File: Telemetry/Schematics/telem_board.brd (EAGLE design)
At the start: 39.9 x 66 mm, 30 parts, among them IC1 PIC18F26K80I/SP, IC2 PTN78000WAH, IC3 ISO1050DUB, IC4 FT232RL, J1 ICD, J2 TELEM, J3 TELEM, J4 TEMP SENSOR, J5 HALL SENSOR, Q4 20M, X1 PN61729-S, X2 +12V

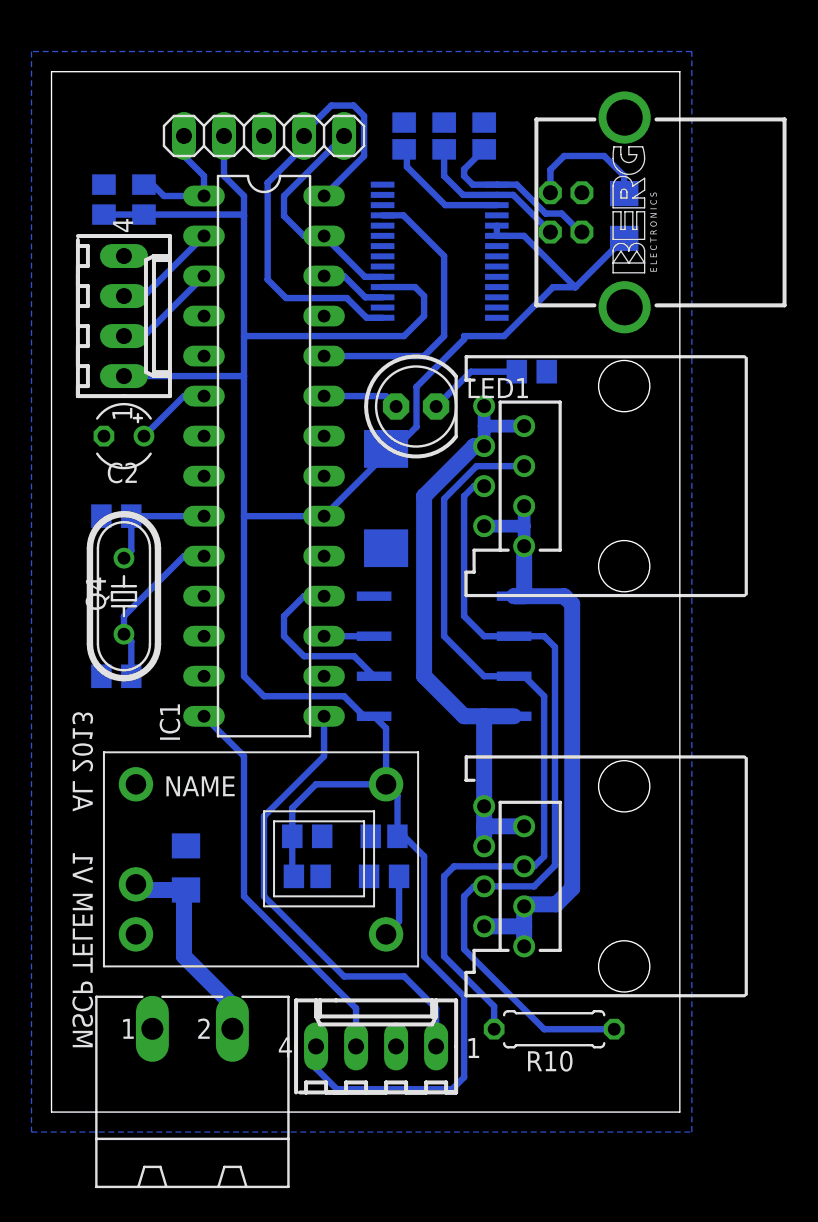
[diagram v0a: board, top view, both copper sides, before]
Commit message: v2
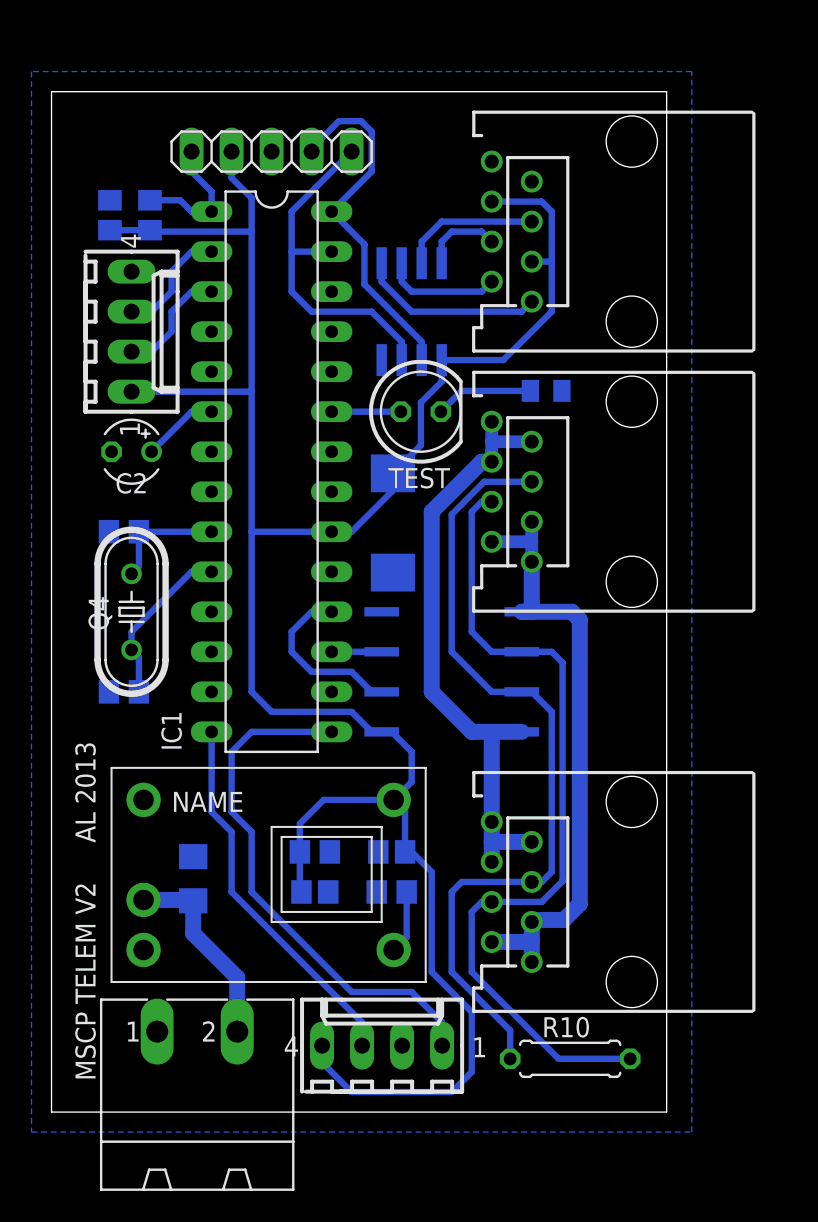
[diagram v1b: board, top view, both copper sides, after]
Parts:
- removed C10: 100n, resistor:C0805
- removed C3, C8: 47p, resistor:C0805
- removed F1: 0.5, MSCP_2011_v2:F1206
- removed LED1: (no value), adafruit:LED5MM
- removed X2: +12V, con-phoenix-508:MSTBA2
- added J7: RADIO, con-amp:215877-7
- added TEST: (no value), led:LED5MM
- IC4: value FT232RL -> SN75LBC179D; device MSCP_2011_v2:SSOP28 -> MSCP_2011_v1:SO08
- J2, J3: value TELEM -> CANBUS
- R2: device rcl:R0805 -> adafruit:R0805
- X1: value PN61729-S -> +12V; device con-berg:PN61729-S -> con-phoenix-508:MSTBA2
- moved X1 63.2 mm to (9.25, 0.03), turned to 0 degrees
- moved IC4 4.23 mm to (22.9, 50.8), turned to 0 degrees
- moved R10 2.14 mm to (32.9, 3.38)
- moved C4 1.61 mm to (21.7, 37.4)
- moved R2 1.52 mm to (31.4, 45.8), turned to 0 degrees
- moved IC1 1.10 mm to (14.0, 40.6)
- moved J1 1.10 mm to (14.0, 61.0)
- moved C7 1.10 mm to (4.60, 36.8)
- moved C2 1.10 mm to (5.08, 41.9)
- moved J4 1.10 mm to (5.08, 49.5)
- moved Q4 1.10 mm to (5.08, 31.8)
- moved C11 1.10 mm to (16.7, 14.0)
- moved IC2 1.10 mm to (14.0, 15.2)
- moved J2 1.10 mm to (36.8, 39.4)
- moved R1 1.10 mm to (21.6, 14.0)
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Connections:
- removed net N$9: C10.1, IC4.17
- new net N$12: IC4.5, J7.1
- net +12V: now also X1.2; no longer X2.2
- net +5V: now also IC4.1, J7.3, J7.6; no longer F1.1, IC4.19, IC4.20, IC4.4
- net CTS: no longer IC4.11
- net GND: now also IC4.4, J7.7, J7.8, R2.1, X1.1; no longer C10.2, C3.2, C8.2, IC4.18, IC4.21, IC4.25, IC4.26, IC4.7, R2.2, X1.4, X2.1
- net N$10: now also IC4.6, J7.2; no longer F1.2, X1.1
- net N$3: now also IC4.7, J7.5; no longer IC1.23, LED1.A
- net N$4: now also IC4.8, J7.4; no longer LED1.K, R2.1
- net N$6: now also IC1.23, TEST.A; no longer C8.1, IC4.16, X1.2
- net N$7: now also R2.2, TEST.K; no longer C3.1, IC4.15, X1.3
- net RTS: no longer IC4.3
- net RX: now also IC4.2; no longer IC4.1
- net TX: now also IC4.3; no longer IC4.5
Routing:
- net CTS: track 18.2 -> 0.00 mm
- net +5V: track 165.4 -> 148.7 mm
- net N$12: track 0.00 -> 11.7 mm
- net TX: track 14.5 -> 22.5 mm
- net N$9: track 7.90 -> 0.00 mm
- net RX: track 29.5 -> 22.9 mm
- net N$6: track 9.91 -> 4.39 mm
- net N$7: track 11.2 -> 6.23 mm
- net RTS: track 4.27 -> 0.00 mm
- net N$3: track 4.85 -> 8.88 mm
- net SDA: track 29.3 -> 33.3 mm
- net N$15: track 51.2 -> 52.3 mm
- net N$14: track 50.6 -> 51.8 mm
- net SCL: track 25.0 -> 23.9 mm
- net +12V: track 13.7 -> 12.6 mm
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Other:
- board size 39.9 x 66 mm -> 39 x 64.8 mm
- board text added: "MSCP TELEM V2 AL 2013"
- board text removed: "MSCP TELEM V1 AL 2013"

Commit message: v3
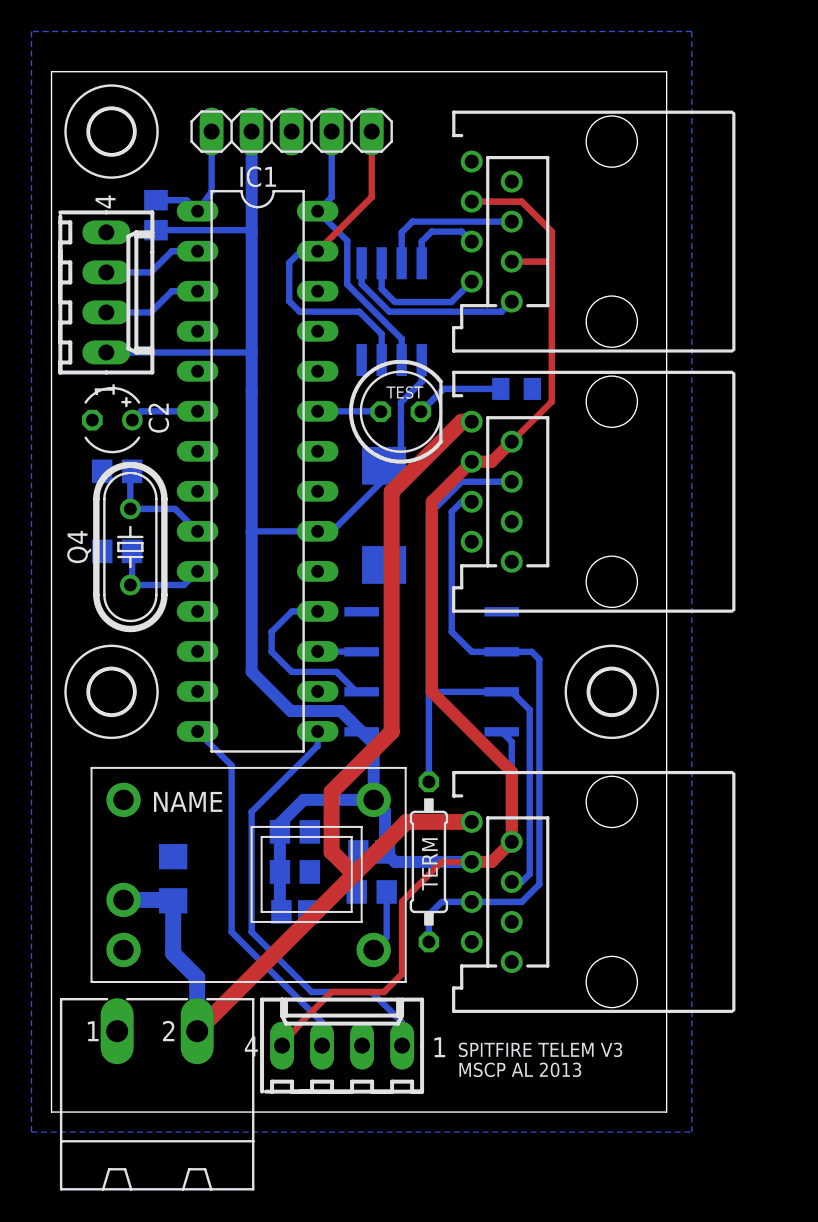
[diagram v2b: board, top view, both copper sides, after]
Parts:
- removed R10: 100, rcl:0207/7
- added H2, H3, H4: MOUNT-HOLE2.8, holes:2,8
- added TERM: 100, resistor:0207/10
- J4: value TEMP SENSOR -> HALLSENS
- J5: value HALL SENSOR -> TEMPSENS
- moved C5 43.3 mm to (15.4, 15.2), turned to 180 degrees
- moved C9 8.93 mm to (4.17, 35.6)
- moved Q4 4.12 mm to (5.00, 35.9)
- moved C7 3.86 mm to (4.17, 40.7)
- moved J4 2.96 mm to (3.48, 52.0)
- moved X1 2.54 mm to (6.71, 0.05)
- moved J5 2.54 mm to (18.4, 4.22)
- moved C2 2.35 mm to (3.86, 43.9)
- moved R2 1.88 mm to (29.5, 45.9)
- moved C11 1.80 mm to (15.4, 12.7)
- moved C6 1.80 mm to (15.4, 17.8)
- moved J1 1.80 mm to (15.2, 62.2)
- moved IC2 1.27 mm to (12.7, 15.2)
- moved C1 1.27 mm to (7.72, 14.8)
- moved C12 1.27 mm to (20.3, 16.5)
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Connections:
- removed net N$14: IC3.7, J2.5, J3.5, R10.2
- removed net N$15: IC3.6, J2.4, J3.4, R10.1
- removed net N$16: IC3.5, J2.1, J2.2, J2.3, J3.1, J3.2, J3.3
- removed net N$32: IC3.8, J2.6, J2.7, J2.8, J3.6, J3.7, J3.8
- new net CANH: IC3.7, J2.5, J3.5, TERM.1
- new net CANL: IC3.6, J2.4, J3.4, TERM.2
- net +12V: now also J2.8, J3.8
- net +5V: now also IC3.8, J2.6, J2.7, J3.6, J3.7
- net GND: now also IC3.5, J2.1, J2.2, J2.3, J3.1, J3.2, J3.3
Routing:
- net +12V: track 12.6 -> 68.4 mm
- net N$15: track 52.3 -> 0.00 mm
- net N$14: track 51.8 -> 0.00 mm
- net CANH: track 0.00 -> 41.7 mm
- net N$32: track 39.8 -> 0.00 mm
- net N$16: track 39.4 -> 0.00 mm
- net CANL: track 0.00 -> 39.3 mm
- net +5V: track 148.7 -> 187.1 mm
- net RX: track 22.9 -> 17.1 mm
- net SDA: track 33.3 -> 27.9 mm
- net N$25: track 10.7 -> 6.80 mm
- net N$1: track 7.40 -> 6.35 mm
- net N$2: track 7.40 -> 6.35 mm
- net N$10: track 7.41 -> 8.22 mm
- net SCL: track 23.9 -> 23.2 mm
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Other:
- board size 39 x 64.8 mm -> 39 x 66 mm
- board text added: "MSCP AL 2013"
- board text added: "SPITFIRE TELEM V3"
- board text removed: "MSCP TELEM V2 AL 2013"
